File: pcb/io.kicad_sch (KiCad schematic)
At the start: 25 parts

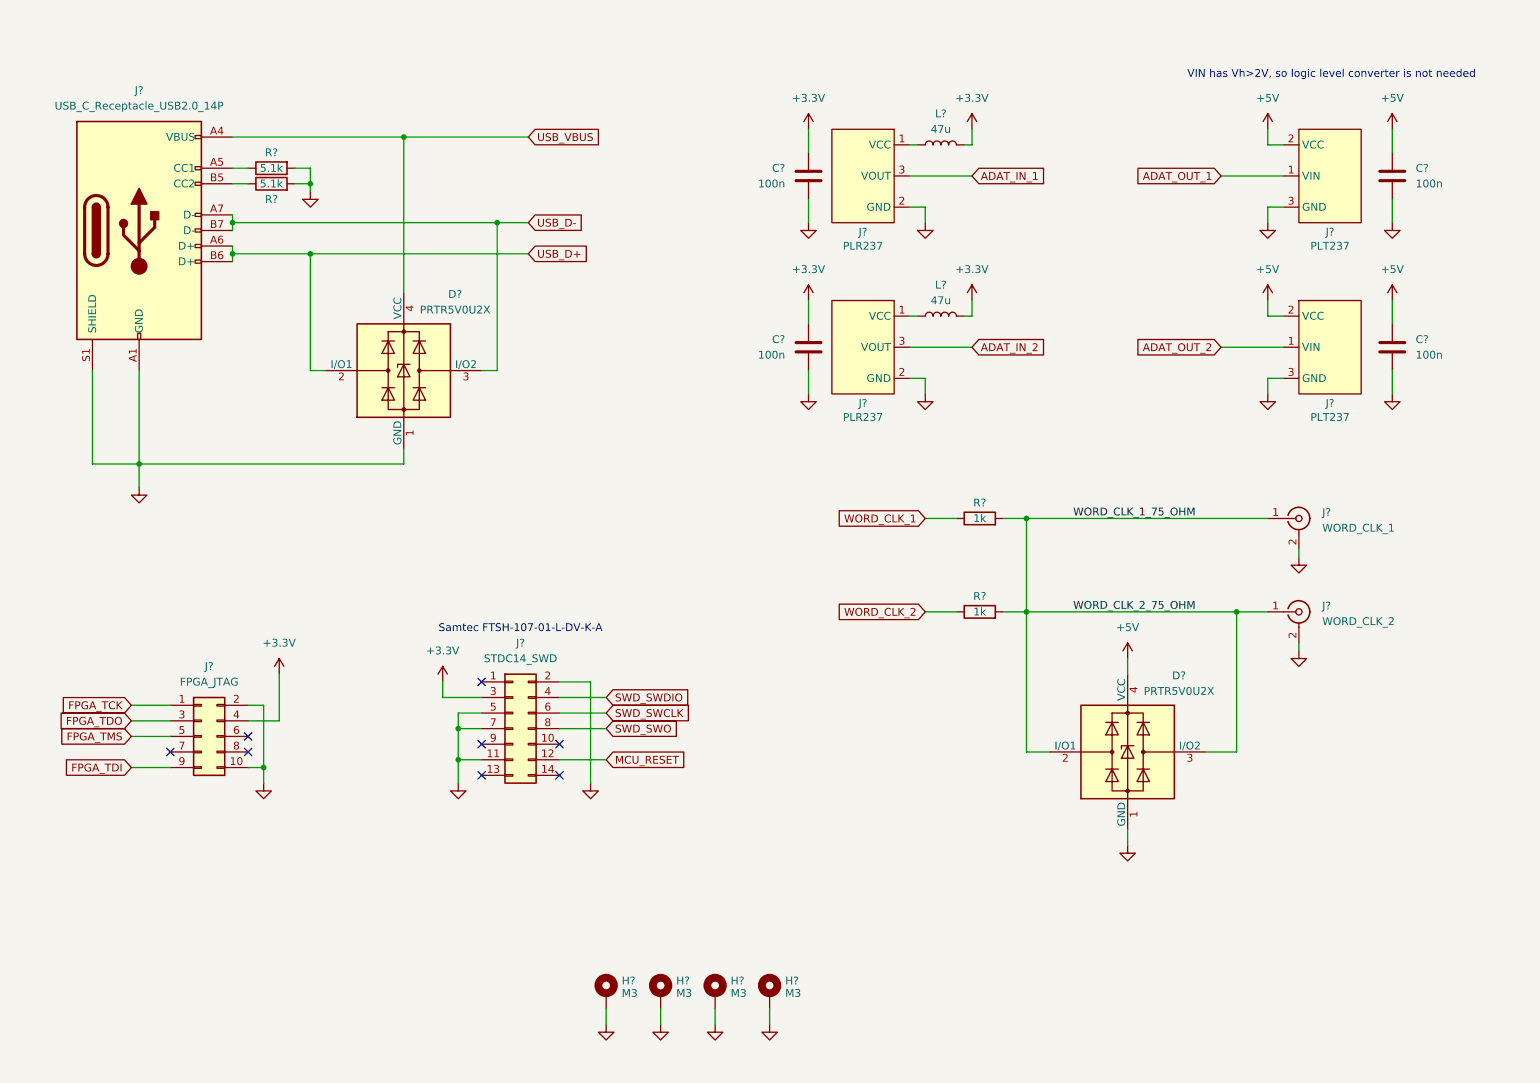
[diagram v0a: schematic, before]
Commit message: Further schematic capture
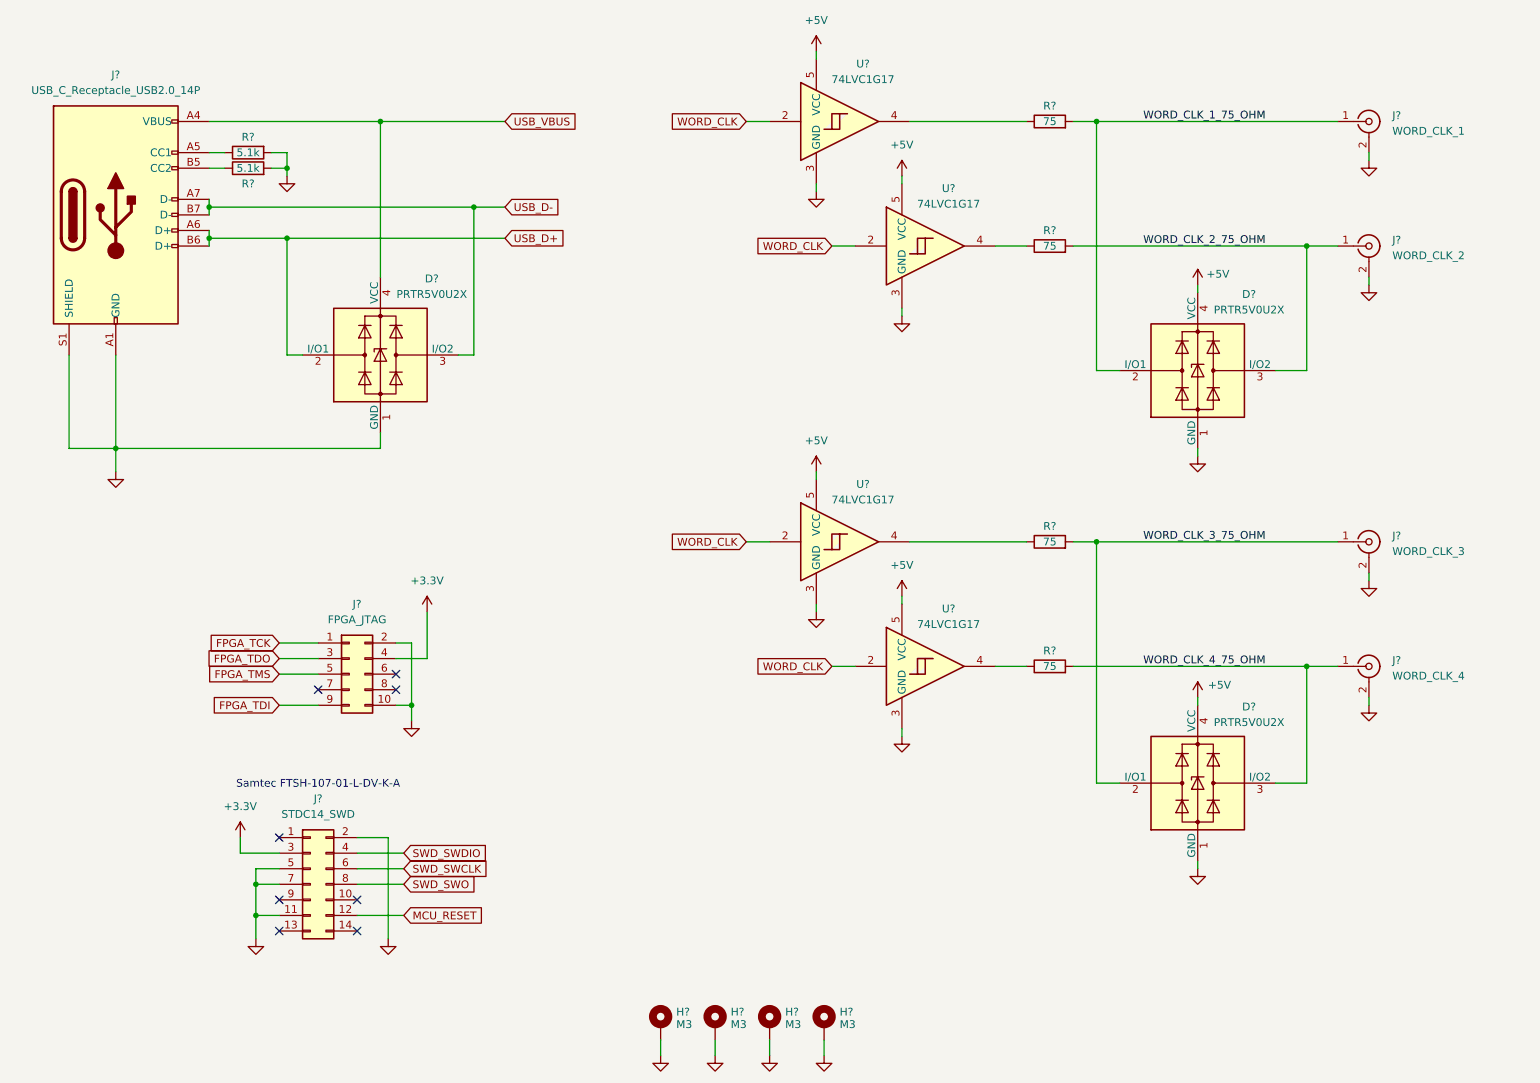
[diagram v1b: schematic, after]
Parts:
- removed C? (x4): 100n, symbol Device:C
- removed J? (x2): PLR237, adatv2:PLx237, symbol adatv2:PLR237
- removed J? (x2): PLT237, adatv2:PLx237, symbol adatv2:PLT237
- removed L? (x2): 47u, symbol Device:L
- added D?: PRTR5V0U2X, Package_TO_SOT_SMD:SOT-143, symbol Power_Protection:PRTR5V0U2X
- added J?: WORD_CLK_4, symbol Connector:Conn_Coaxial
- added J?: WORD_CLK_3, symbol Connector:Conn_Coaxial
- added R? (x2): 75, symbol Device:R
- added U? (x4): 74LVC1G17, Package_TO_SOT_SMD:SOT-23-5, symbol 74xGxx:74LVC1G17
- R? (x2): value 1k -> 75
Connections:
- net +5V: now also D?.4 (VCC), U?.5 (VCC), U?.5 (VCC), U?.5 (VCC), U?.5 (VCC)
- net GND: now also D?.1 (GND), J?.2 (Ext), J?.2 (Ext), U?.3 (GND), U?.3 (GND), U?.3 (GND), U?.3 (GND)
- net WORD_CLK_1_75_OHM: no longer D?.3 (I/O2), J?.1 (In), R?.2
- net WORD_CLK_1: no longer names the net of R?.1
- net WORD_CLK_1: now also U?.4
- net WORD_CLK_2: no longer names the net of R?.1
- net WORD_CLK_2: now also U?.4
- new net: R?.1, U?.4 (x2)
- new net WORD_CLK: U?.2, U?.2, U?.2, U?.2
- new net WORD_CLK_2_75_OHM: D?.3 (I/O2), J?.1 (In), R?.2
- new net WORD_CLK_3_75_OHM: D?.2 (I/O1), J?.1 (In), R?.2
- new net WORD_CLK_4_75_OHM: D?.3 (I/O2), J?.1 (In), R?.2
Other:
- note removed: "VIN has Vh>2V, so logic level converter is not needed"
- moved on the sheet: D?, H?, J?, R?

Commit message: Further schematic capture
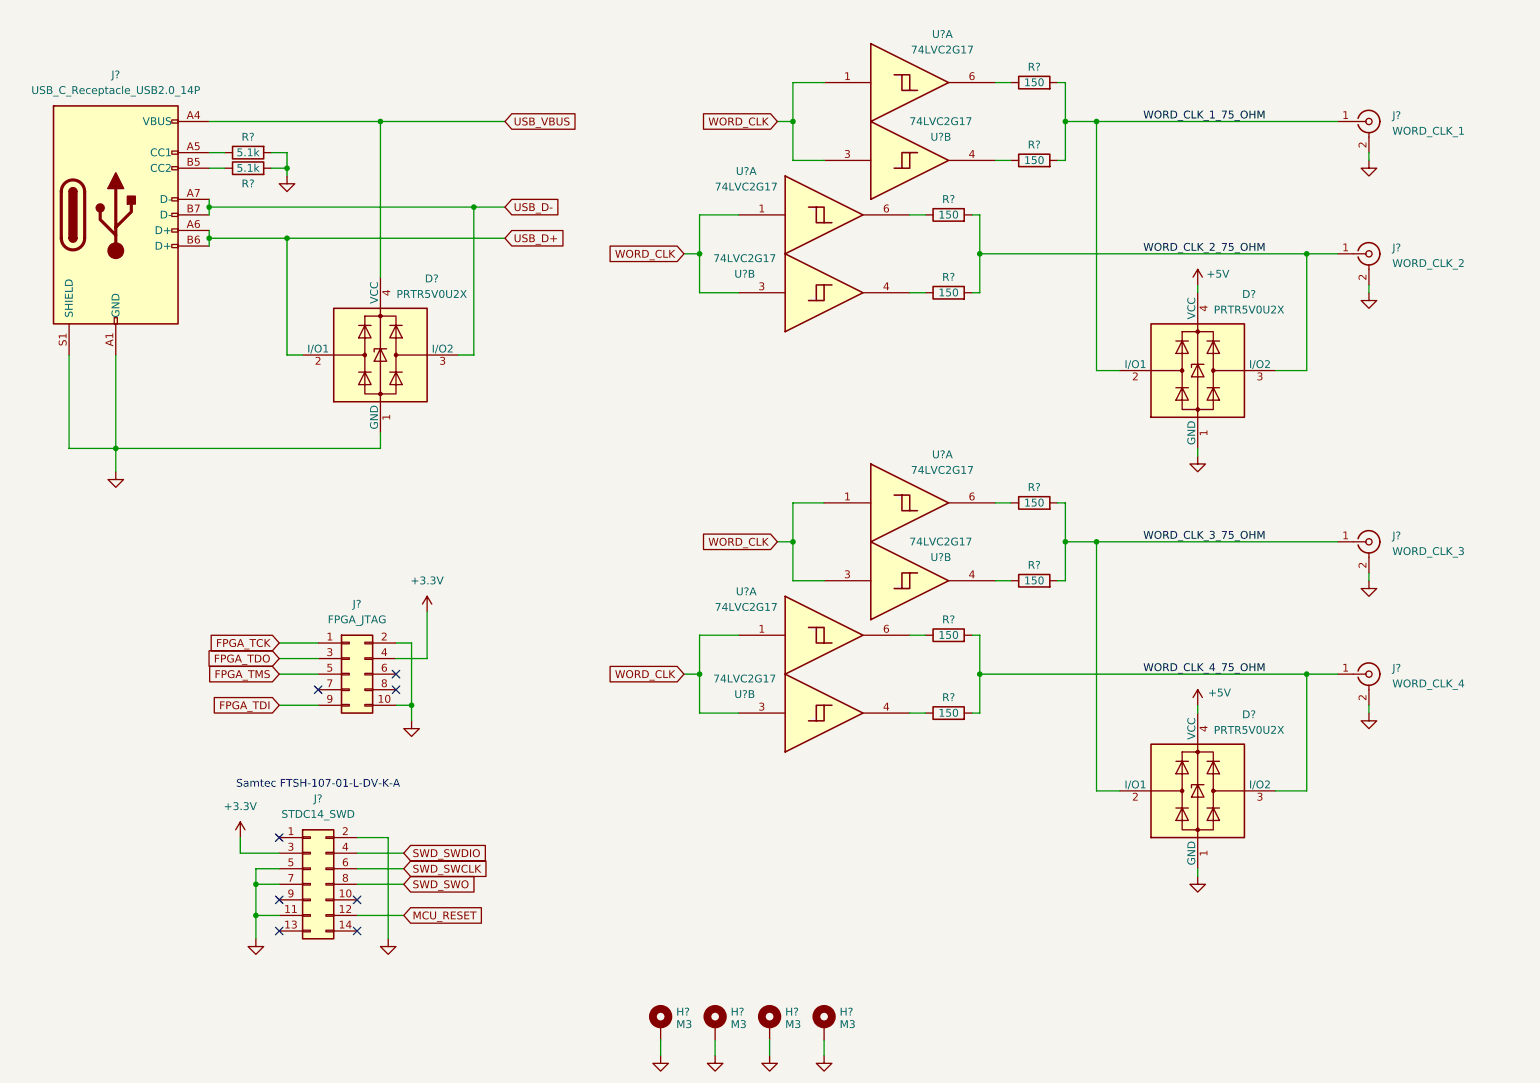
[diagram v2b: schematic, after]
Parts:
- removed R? (x3): 75, symbol Device:R
- removed U? (x4): 74LVC1G17, Package_TO_SOT_SMD:SOT-23-5, symbol 74xGxx:74LVC1G17
- added R? (x7): 150, symbol Device:R
- added U? (x8): 74LVC2G17, symbol 74xGxx:74LVC2G17
- R?: value 75 -> 150
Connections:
- net WORD_CLK: now also U?.1, U?.1, U?.1, U?.1, U?.3, U?.3, U?.3, U?.3
- net WORD_CLK_1_75_OHM: now also R?.2
- net WORD_CLK_2_75_OHM: now also R?.2, R?.2
- net WORD_CLK_3_75_OHM: now also R?.2, R?.2
- net WORD_CLK_4_75_OHM: now also R?.2, R?.2
- net at R?.1: now also U?.6
- new net: R?.1, U?.4 (x4)
- new net: R?.1, U?.6 (x3)
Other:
- moved on the sheet: D?, J?, R?
